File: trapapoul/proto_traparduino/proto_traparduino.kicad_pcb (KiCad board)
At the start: 2 copper layers, 68.6 x 53.3 mm, 8 parts, among them P1 Power, P2 Analog, P3 Digital, P4 Digital, P5 CONN_1, P6 CONN_1, P7 CONN_1, P8 CONN_1

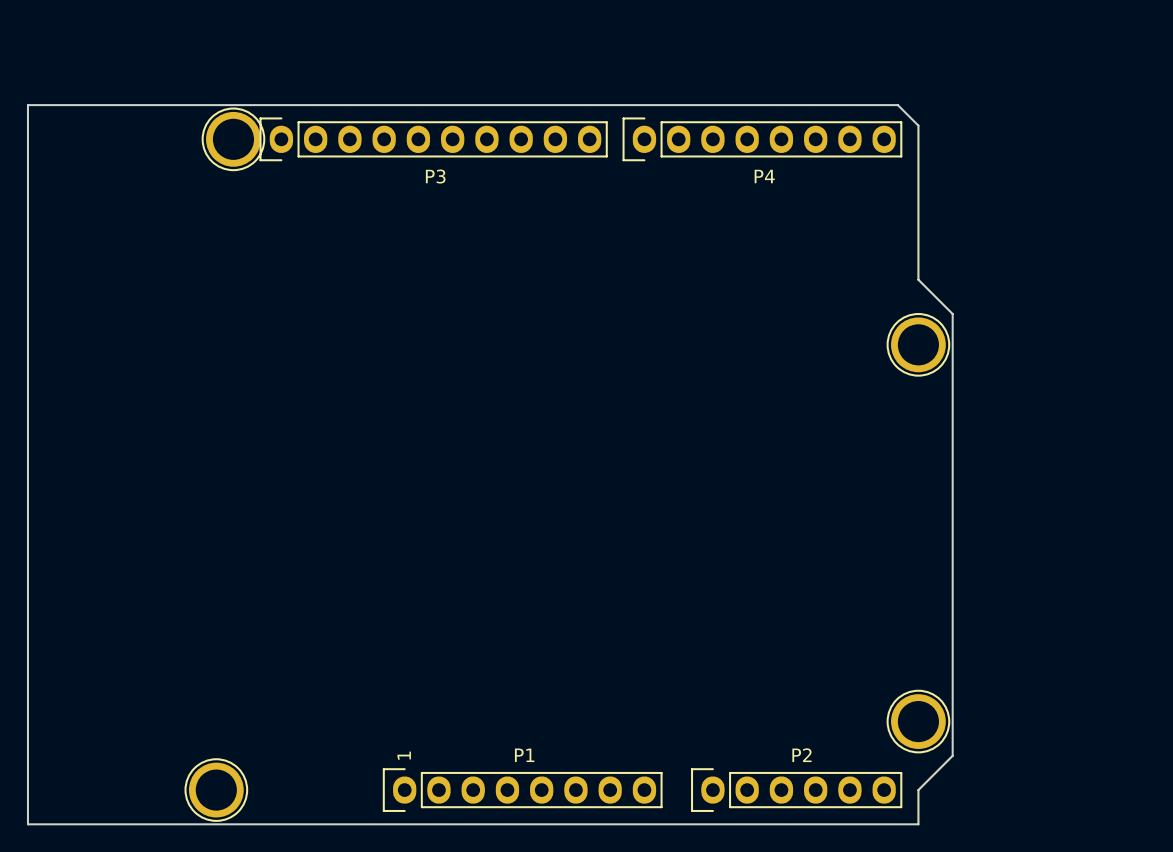
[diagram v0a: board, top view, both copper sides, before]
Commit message: trapapoul_proto2 fini
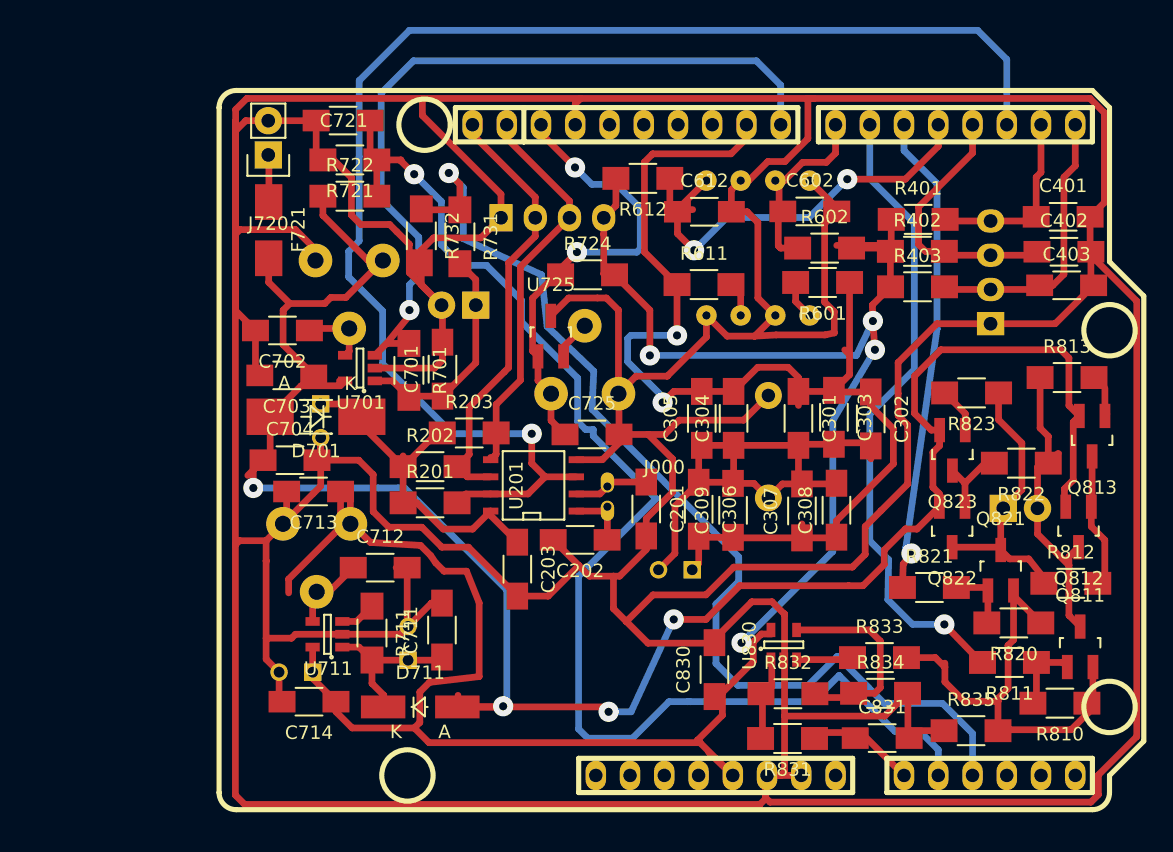
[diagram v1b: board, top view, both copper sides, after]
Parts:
- removed P1: Power, Socket_Arduino_Uno:Socket_Strip_Arduino_1x08
- removed P2: Analog, Socket_Arduino_Uno:Socket_Strip_Arduino_1x06
- removed P3: Digital, Socket_Arduino_Uno:Socket_Strip_Arduino_1x10
- removed P4: Digital, Socket_Arduino_Uno:Socket_Strip_Arduino_1x08
- removed P5, P6, P7, P8: CONN_1, Socket_Arduino_Uno:Arduino_1pin
- added C201: 10p, Capacitors_SMD:C_1206_HandSoldering, F.Cu at (156.8, 103.0)
- added C202: 10p, Capacitors_SMD:C_1206_HandSoldering, F.Cu at (151.9, 105.3)
- added C203: 10n, Capacitors_SMD:C_1206_HandSoldering, F.Cu at (147.3, 107.4)
- added C301: 10uF, Capacitors_SMD:C_1206_HandSoldering, F.Cu at (168.1, 96.3)
- added C302: 10uF, Capacitors_SMD:C_1206_HandSoldering, F.Cu at (173.5, 96.3)
- added C303: 10uF, Capacitors_SMD:C_1206_HandSoldering, F.Cu at (170.8, 96.2)
- added C304: 10uF, Capacitors_SMD:C_1206_HandSoldering, F.Cu at (163.3, 96.3)
- added C305: 10uF, Capacitors_SMD:C_1206_HandSoldering, F.Cu at (161.0, 96.3)
- added C306: 10uF, Capacitors_SMD:C_1206_HandSoldering, F.Cu at (160.7, 103.0)
- added C307: 10uF, Capacitors_SMD:C_1206_HandSoldering, F.Cu at (168.4, 103.1)
- added C308: 10uF, Capacitors_SMD:C_1206_HandSoldering, F.Cu at (171.0, 103.1)
- added C309: 10uF, Capacitors_SMD:C_1206_HandSoldering, F.Cu at (163.3, 103.1)
- added C310: 220u, Capacitors_ThroughHole:C_Radial_D7.5_L11.2_P2.5, B.Cu at (160.3, 107.5)
- added C401: 10n, Capacitors_SMD:C_1206_HandSoldering, F.Cu at (187.8, 81.3)
- added C402: 10n, Capacitors_SMD:C_1206_HandSoldering, F.Cu at (187.8, 83.9)
- added C403: 10n, Capacitors_SMD:C_1206_HandSoldering, F.Cu at (188.0, 86.4)
- added C602: 100nF, Capacitors_SMD:C_1206_HandSoldering, F.Cu at (169.0, 80.9)
- added C612: 100nF, Capacitors_SMD:C_1206_HandSoldering, F.Cu at (161.2, 80.9)
- added C701: 10u, Capacitors_SMD:C_1206_HandSoldering, F.Cu at (141.7, 92.6)
- added C702: 1n, Capacitors_SMD:C_1206_HandSoldering, F.Cu at (129.9, 89.7)
- added C703: 100n, Capacitors_SMD:C_1206_HandSoldering, F.Cu at (130.2, 93.1)
- added C704: 10u, Capacitors_SMD:C_1206_HandSoldering, F.Cu at (130.4, 99.4)
- added C705: 220u, Capacitors_ThroughHole:C_Radial_D7.5_L11.2_P2.5, B.Cu at (132.7, 95.2)
- added C710: 220u, Capacitors_ThroughHole:C_Radial_D7.5_L11.2_P2.5, B.Cu at (139.2, 114.2)
- added C711: 10u, Capacitors_SMD:C_1206_HandSoldering, F.Cu at (141.7, 112.0)
- added C712: 1n, Capacitors_SMD:C_1206_HandSoldering, F.Cu at (137.1, 107.3)
- added C713: 100n, Capacitors_SMD:C_1206_HandSoldering, F.Cu at (132.2, 101.7)
- added C714: 10u, Capacitors_SMD:C_1206_HandSoldering, F.Cu at (131.8, 117.3)
- added C715: 220u, Capacitors_ThroughHole:C_Radial_D7.5_L11.2_P2.5, B.Cu at (132.1, 115.1)
- added C721: 10n, Capacitors_SMD:C_1206_HandSoldering, F.Cu at (134.4, 74.2)
- added C725: 10n, Capacitors_SMD:C_1206_HandSoldering, F.Cu at (152.8, 97.5)
- added C830: 100n, Capacitors_SMD:C_1206_HandSoldering, F.Cu at (161.9, 114.9)
- added C831: 100n, Capacitors_SMD:C_1206_HandSoldering, F.Cu at (174.3, 120.0)
- added D701: SCHOTTKY, Diodes_SMD:MELF_Handsoldering, F.Cu at (132.4, 96.1)
- added D711: SCHOTTKY, Diodes_SMD:MiniMELF_Handsoldering, F.Cu at (140.1, 117.7)
- added F721: 5A, Fuse_Holders_and_Fuses:Fuse_SMD1206_HandSoldering, F.Cu at (128.8, 82.3)
- added J000: Arduino_Header, w_conn_misc:arduino_header, F.Cu at (158.2, 98.6)
- added J400: HEADER_4, Pin_Headers:Pin_Header_Straight_1x04, B.Cu at (182.4, 89.2)
- added J720: HEADER_2, Pin_Headers:Pin_Header_Straight_1x02, F.Cu at (128.8, 76.7)
- added J730: HEADER_2, Pin_Headers:Pin_Header_Straight_1x02, B.Cu at (144.2, 87.9)
- added J740: HEADER_4, Pin_Headers:Pin_Header_Straight_1x04, B.Cu at (146.1, 81.4)
- added J800: HEADER_2, Pin_Headers:Pin_Header_Straight_1x02, B.Cu at (183.3, 102.9)
- added Q811: PBSS4320, TO_SOT_Packages_SMD:SOT-23_Handsoldering, F.Cu at (189.0, 113.2)
- added Q812: PBSS5350, TO_SOT_Packages_SMD:SOT-23_Handsoldering, F.Cu at (188.9, 104.3)
- added Q813: PBSS5350, TO_SOT_Packages_SMD:SOT-23_Handsoldering, F.Cu at (189.9, 97.6)
- added Q821: PBSS4320, TO_SOT_Packages_SMD:SOT-23_Handsoldering, F.Cu at (183.1, 107.5)
- added Q822: PBSS5350, TO_SOT_Packages_SMD:SOT-23_Handsoldering, F.Cu at (179.5, 104.3)
- added Q823: PBSS5350, TO_SOT_Packages_SMD:SOT-23_Handsoldering, F.Cu at (179.6, 98.6)
- added R201: 10k, Resistors_SMD:R_1206_HandSoldering, F.Cu at (140.8, 102.5)
- added R202: 2.2k, Resistors_SMD:R_1206_HandSoldering, F.Cu at (140.8, 99.8)
- added R203: 2.2k, Resistors_SMD:R_1206_HandSoldering, F.Cu at (143.7, 97.3)
- added R401: 10k, Resistors_SMD:R_1206_HandSoldering, F.Cu at (177.0, 81.5)
- added R402: 10k, Resistors_SMD:R_1206_HandSoldering, F.Cu at (177.0, 83.9)
- added R403: 10k, Resistors_SMD:R_1206_HandSoldering, F.Cu at (177.0, 86.5)
- added R601: 220, Resistors_SMD:R_1206_HandSoldering, F.Cu at (169.9, 86.2)
- added R602: 4k7, Resistors_SMD:R_1206_HandSoldering, F.Cu at (170.1, 83.6)
- added R611: 220, Resistors_SMD:R_1206_HandSoldering, F.Cu at (161.1, 86.3)
- added R612: 4k7, Resistors_SMD:R_1206_HandSoldering, F.Cu at (156.6, 78.5)
- added R701: 10k, Resistors_SMD:R_1206_HandSoldering, F.Cu at (139.2, 92.7)
- added R711: 10k, Resistors_SMD:R_1206_HandSoldering, F.Cu at (136.5, 112.2)
- added R721: 10k, Resistors_SMD:R_1206_HandSoldering, F.Cu at (134.9, 77.1)
- added R722: 10k, Resistors_SMD:R_1206_HandSoldering, F.Cu at (134.9, 79.8)
- added R724: 10k, Resistors_SMD:R_1206_HandSoldering, F.Cu at (152.5, 85.6)
- added R731: 10k, Resistors_SMD:R_1206_HandSoldering, F.Cu at (143.0, 82.8)
- added R732: 10k, Resistors_SMD:R_1206_HandSoldering, F.Cu at (140.2, 82.7)
- added R810: 330, Resistors_SMD:R_1206_HandSoldering, F.Cu at (187.5, 117.4)
- added R811: 330, Resistors_SMD:R_1206_HandSoldering, F.Cu at (183.8, 114.4)
- added R812: 330, Resistors_SMD:R_1206_HandSoldering, F.Cu at (188.3, 108.5)
- added R813: 3k3, Resistors_SMD:R_1206_HandSoldering, F.Cu at (188.1, 93.2)
- added R820: 330, Resistors_SMD:R_1206_HandSoldering, F.Cu at (184.1, 111.4)
- added R821: 330, Resistors_SMD:R_1206_HandSoldering, F.Cu at (177.8, 108.8)
- added R822: 330, Resistors_SMD:R_1206_HandSoldering, F.Cu at (184.7, 99.6)
- added R823: 3k3, Resistors_SMD:R_1206_HandSoldering, F.Cu at (181.0, 94.4)
- added R831: 1k, Resistors_SMD:R_1206_HandSoldering, F.Cu at (167.3, 120.0)
- added R832: 10k, Resistors_SMD:R_1206_HandSoldering, F.Cu at (167.4, 116.7)
- added R833: 1k, Resistors_SMD:R_1206_HandSoldering, F.Cu at (174.2, 114.0)
- added R834: 1k, Resistors_SMD:R_1206_HandSoldering, F.Cu at (174.2, 116.7)
- added R835: 0R2, Resistors_SMD:R_1206_HandSoldering, F.Cu at (180.9, 119.4)
- added RP70: 100k, Potentiometers:Potentiometer_Triwood_RM-065, B.Cu at (132.3, 84.5)
- added RP71: 100k, Potentiometers:Potentiometer_Triwood_RM-065, B.Cu at (129.9, 104.1)
- added RP72: 10k, Potentiometers:Potentiometer_Triwood_RM-065, B.Cu at (154.8, 94.4)
- added U201: MCP7940, SMD_Packages:SOIC-8-N, F.Cu at (148.5, 101.2)
- added U300: buzzer, Buzzers_Beepers:Buzzer_12x9.5RM7.6, B.Cu at (165.9, 98.4)
- added U601: ITR9606, gdi:ITR9606, B.Cu at (167.7, 83.6)
- added U611: ITR9606, gdi:ITR9606, B.Cu at (162.6, 83.6)
- added U701: MIC5205, TO_SOT_Packages_SMD:SOT-23-5, F.Cu at (135.6, 92.5)
- added U711: MIC5205, TO_SOT_Packages_SMD:SOT-23-5, F.Cu at (133.2, 112.3)
- added U725: TLV431-DBZ, TO_SOT_Packages_SMD:SOT-23_Handsoldering, F.Cu at (149.8, 90.2)
- added U830: MCP601-SOT, TO_SOT_Packages_SMD:SOT-23-5, F.Cu at (167.1, 113.0)
- added X201: 32.768K, Crystals:Crystal_Round_Vertical_3mm_BigPad, B.Cu at (154.0, 102.1)
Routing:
- net GND: track 0.00 -> 611.4 mm
- net VCC: track 0.00 -> 165.4 mm, vias 0 -> 4
- net V_bat: track 0.00 -> 156.8 mm, vias 0 -> 4
- net alarm: track 0.00 -> 104.1 mm, vias 0 -> 1
- net M_bat: track 0.00 -> 94.5 mm, vias 0 -> 1
- net buzz: track 0.00 -> 88.3 mm, vias 0 -> 2
- net M_sol: track 0.00 -> 79.3 mm, vias 0 -> 1
- net charge_OFF: track 0.00 -> 58.6 mm, vias 0 -> 1
- net C_frw: track 0.00 -> 47.5 mm, vias 0 -> 1
- net Net-(C301-Pad2): track 0.00 -> 44.2 mm
- net C_bkw: track 0.00 -> 35.9 mm, vias 0 -> 1
- net V_ref: track 0.00 -> 33.5 mm, vias 0 -> 2
- net Net-(Q811-Pad2): track 0.00 -> 33.3 mm
- net quadB: track 0.00 -> 33.1 mm, vias 0 -> 2
- net SCL: track 0.00 -> 33.0 mm
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- added copper zone on F.Cu, net GND
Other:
- board outline removed
- net class Default: clearance 0.2 -> 0.3; trace_width 0.25 -> 0.5; via_dia 0.6 -> 1.5; via_drill 0.4 -> 0.6
- rule trace_clearance: 0.2 -> 0.3
- rule trace_min: 0.2 -> 0.3
- rule via_min_drill: 0.3 -> 0.5
- rule via_min_size: 0.4 -> 1
- board text removed: "1"
